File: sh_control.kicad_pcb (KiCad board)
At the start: 4 copper layers, 77 parts, among them IC1 SN75240PW, IC2 LM317MDCY, IC3 TPS73533DRBT, IC4 TLV76733DGNR, IC5 TUSB2046IBVF, IC6 TPS2044BDR, IC7 SN75240PW, J1 USB_B_Micro, J2 10129381-906001BLF, J3 10129381-906001BLF, J4 USB_A, J5 USB_A, Y1 6MHz

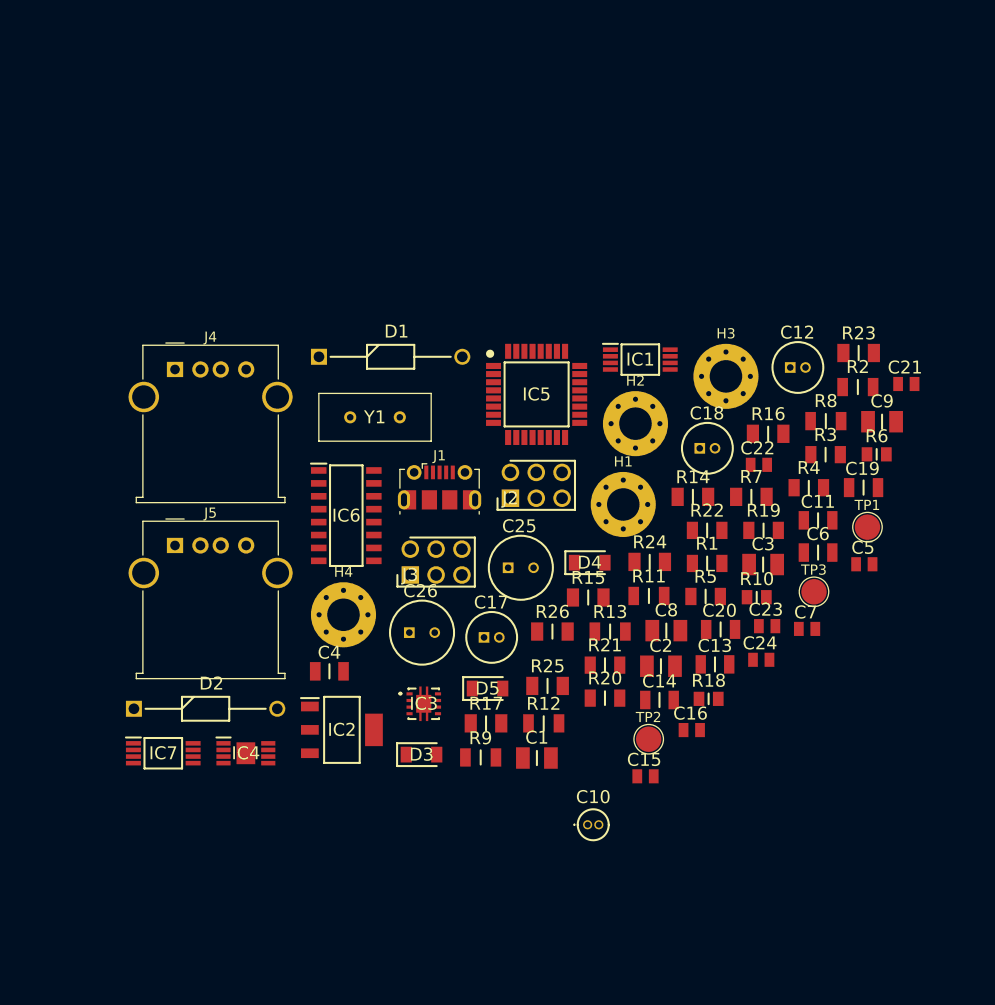
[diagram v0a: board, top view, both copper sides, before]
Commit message: finished schematic, placing parts and so on
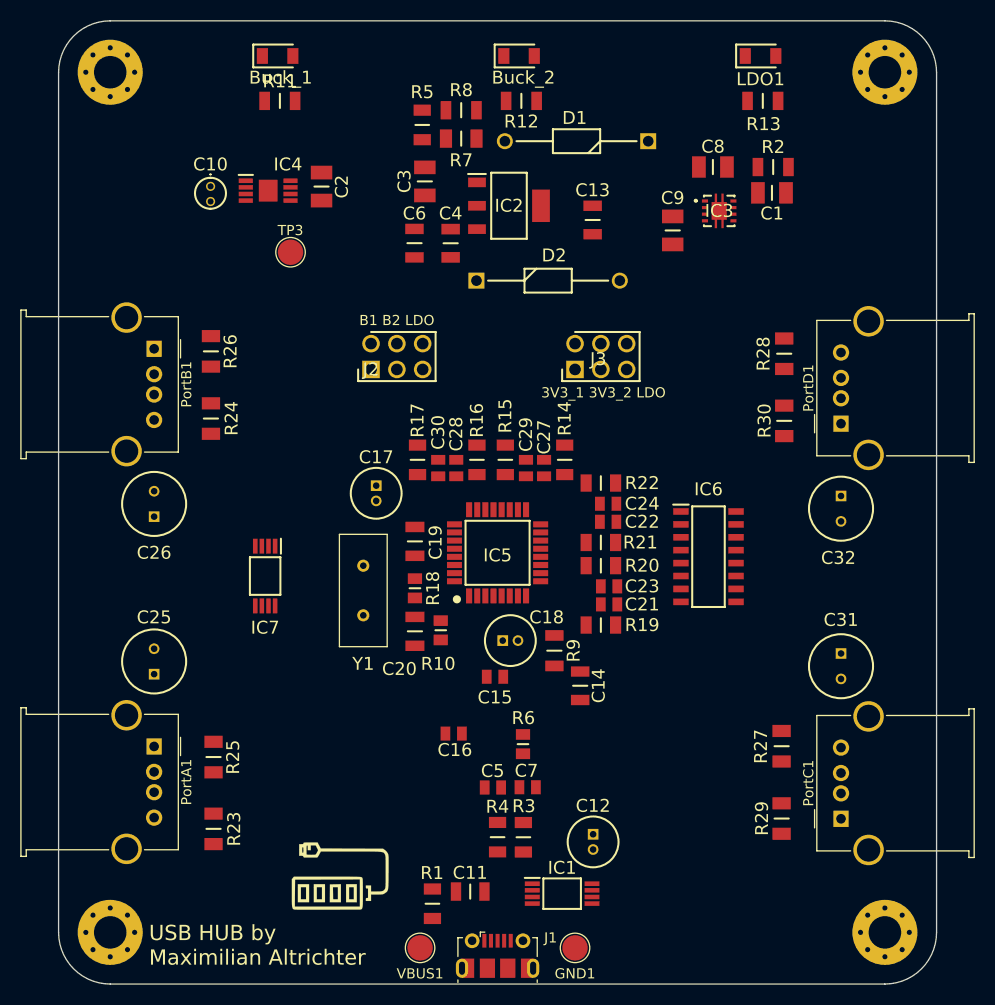
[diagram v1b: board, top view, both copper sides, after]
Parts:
- removed D4: Buck_2, SamacSys_Parts:LEDC3214X78N
- removed D5: LDO, SamacSys_Parts:LEDC3214X78N
- removed J4, J5: USB_A, Connector_USB:USB_A_Molex_67643_Horizontal
- removed TP1: GND, TestPoint:TestPoint_Pad_D2.5mm
- removed TP2: VBUS, TestPoint:TestPoint_Pad_D2.5mm
- added Buck_2: Buck_2, SamacSys_Parts:LEDC3214X78N, F.Cu at (157.1, 36.7)
- added C27: 22pF, storage:C_22pF, F.Cu at (159.5, 77.3)
- added C28: 22pF, storage:C_22pF, F.Cu at (150.9, 77.3)
- added C29: 22pF, storage:C_22pF, F.Cu at (157.7, 77.3)
- added C30: 22pF, storage:C_22pF, F.Cu at (149.1, 77.3)
- added C31: 100uF, storage:C_100uF, F.Cu at (188.7, 95.5)
- added C32: 100uF, storage:C_100uF, F.Cu at (188.7, 80.0)
- added G***: LOGO, logo_hub:logo, F.Cu at (139.4, 117.9)
- added GND1: GND, TestPoint:TestPoint_Pad_D2.5mm, F.Cu at (162.6, 124.5)
- added LDO1: LDO, SamacSys_Parts:LEDC3214X78N, F.Cu at (180.8, 36.7)
- added PortA1: USB_A, Connector_USB:USB_A_Molex_67643_Horizontal, F.Cu at (121.2, 104.6)
- added PortB1: USB_A, Connector_USB:USB_A_Molex_67643_Horizontal, F.Cu at (121.2, 65.5)
- added PortC1: USB_A, Connector_USB:USB_A_Molex_67643_Horizontal, F.Cu at (188.7, 111.8)
- added PortD1: USB_A, Connector_USB:USB_A_Molex_67643_Horizontal, F.Cu at (188.7, 72.9)
- added R27: 15k, storage:R_15K, F.Cu at (182.9, 104.6)
- added R28: 15k, storage:R_15K, F.Cu at (183.1, 66.0)
- added R29: 15k, storage:R_15K, F.Cu at (182.9, 111.7)
- added R30: 15k, storage:R_15K, F.Cu at (183.1, 72.6)
- added VBUS1: VBUS, TestPoint:TestPoint_Pad_D2.5mm, F.Cu at (147.3, 124.5)
- R14, R15, R16, R17: value 15k -> 22; footprint storage:R_15K -> storage:R_22
- moved R23 78.9 mm to (127.0, 112.8), turned to 270 degrees
- moved C10 72.6 mm to (126.7, 50.2), turned to 270 degrees
- moved Buck_1 70.2 mm to (133.3, 36.7)
- moved H2 62.2 mm to (116.8, 38.3)
- moved TP3 61.4 mm to (134.6, 56.0)
- moved R12 61.3 mm to (157.3, 41.1)
- moved R11 60.7 mm to (133.5, 41.1)
- moved C1 60.2 mm to (181.9, 50.2)
- moved C2 57.8 mm to (137.6, 49.6), turned to 270 degrees
- moved IC3 56.5 mm to (176.7, 52.0)
- moved IC4 55.4 mm to (132.4, 50.0)
- moved R13 54.3 mm to (181.0, 41.1)
- moved R5 54.1 mm to (147.5, 43.5), turned to 90 degrees
- moved IC2 54.1 mm to (156.1, 51.5)
- moved D2 53.9 mm to (152.9, 58.8)
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- renumbered D3 to Buck_1
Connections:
- IC1 pad 6: Net-(IC1-Pad6) -> (no net)
- IC1 pad 8: Net-(IC1-Pad8) -> (no net)
- IC3 pad 2: Net-(IC3-Pad2) -> (no net)
- IC3 pad 6: Net-(IC3-Pad6) -> (no net)
- IC3 pad 7: Net-(IC3-Pad7) -> (no net)
- IC4 pad 3: Net-(IC4-Pad3) -> (no net)
- IC4 pad 7: Net-(IC4-Pad7) -> (no net)
- IC5 pad 32: Net-(IC5-Pad32) -> (no net)
- IC5 pad 5: Net-(IC5-Pad5) -> (no net)
- IC6 pad 10: Net-(IC6-Pad10) -> OUT4
- IC6 pad 11: Net-(IC6-Pad11) -> OUT3
- J1 pad 4: Net-(J1-Pad4) -> (no net)
- R14 pad 1: GND -> DM_downstream3
- R14 pad 2: DP3 -> DM3
- R15 pad 1: GND -> DP_downstream3
- R15 pad 2: DM3 -> DP3
- R16 pad 1: GND -> DM_downstream4
- R17 pad 1: GND -> DP_downstream4
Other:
- board outline added: 86.4 x 94.7 mm
- board text added: "3V3_1 3V3_2 LDO"
- board text added: "B1 B2 LDO"
- board text added: "USB HUB by Maximilian Altrichter"
